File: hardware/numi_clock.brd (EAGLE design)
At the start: 70.8 x 29.5 mm, 31 parts, among them IC1 MEGA8-AI, IC2 LM75, Q1 12MHz, Y1 32.768kHz

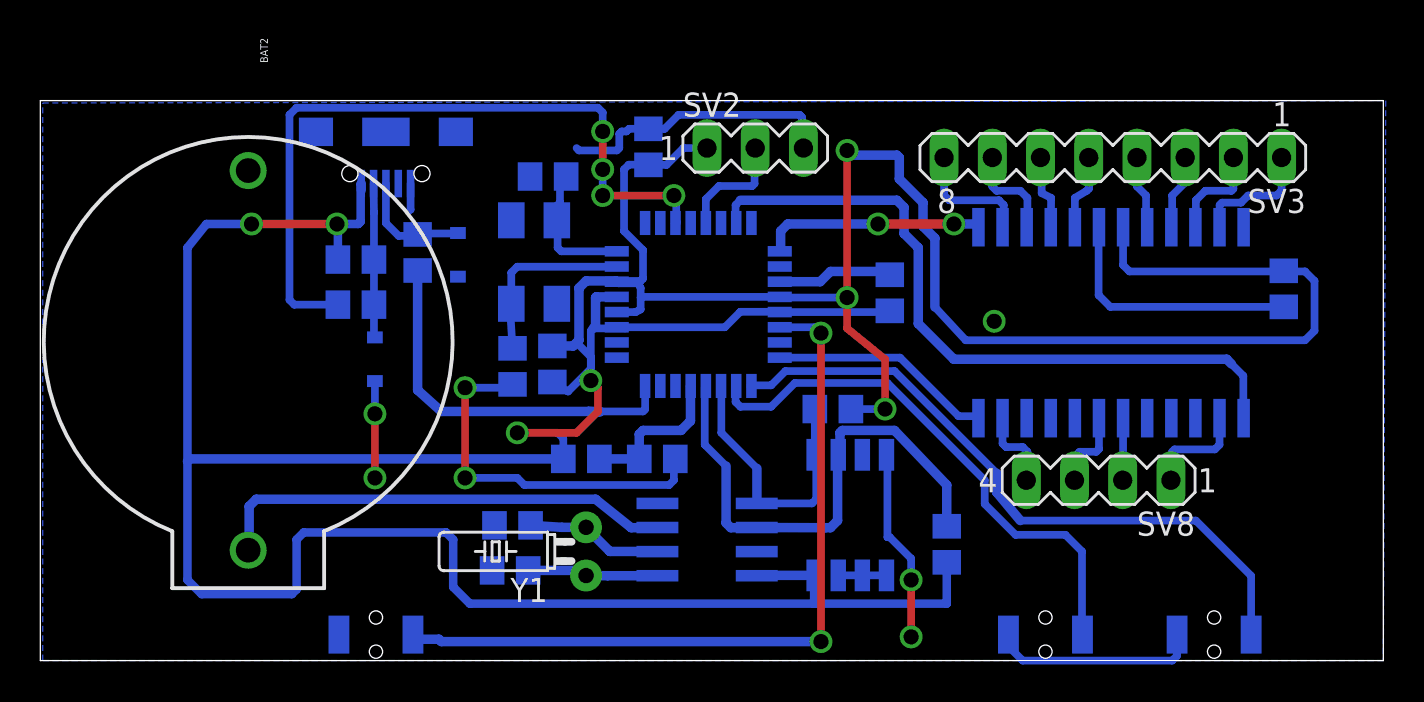
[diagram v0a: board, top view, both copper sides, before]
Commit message: rerouted some tracks
rerouted some tracks
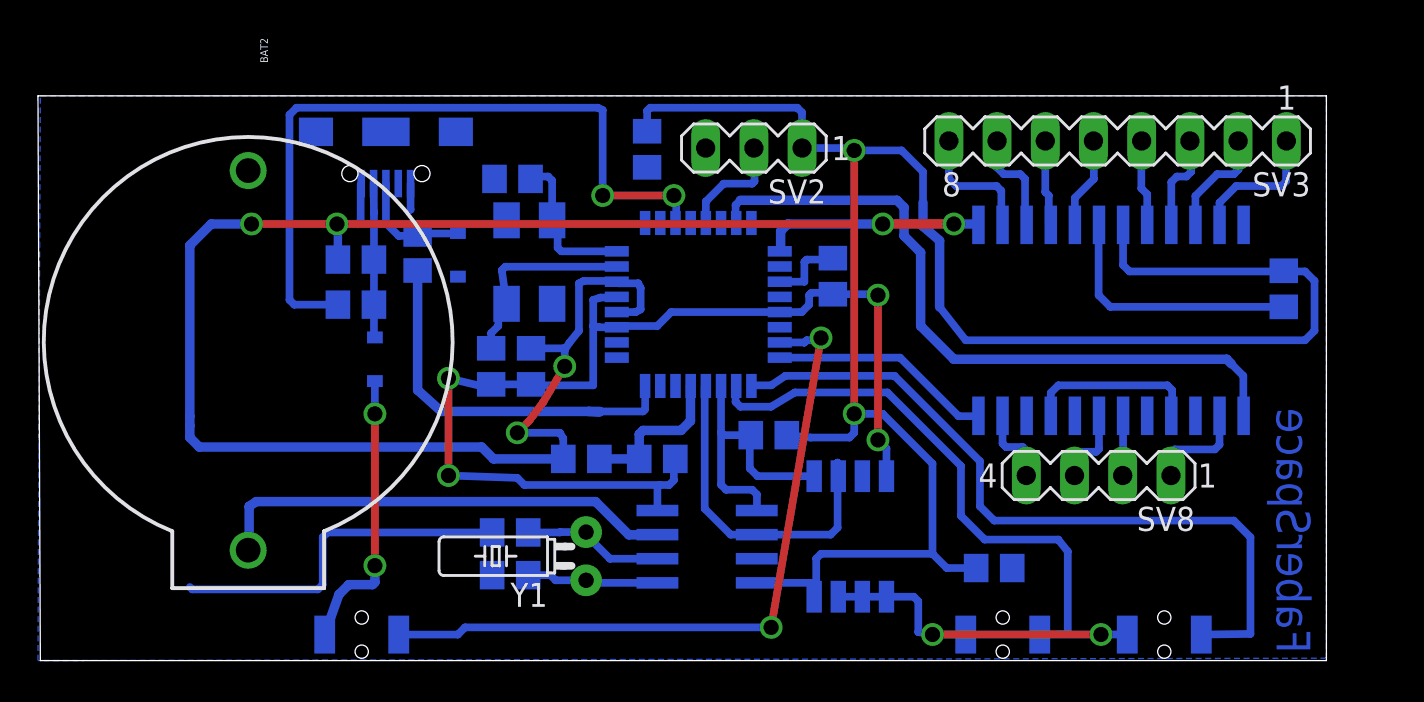
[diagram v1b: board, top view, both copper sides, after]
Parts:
- moved R8 3.64 mm to (53.5, 19.9)
- moved D3 3.12 mm to (56.9, 28.2)
- moved R10 2.80 mm to (65.4, 12.9), turned to 180 degrees
- moved S2 2.62 mm to (74.3, 9.37)
- moved S1 2.25 mm to (65.8, 9.37)
- moved C3 1.88 mm to (40.0, 33.4)
- moved C5 1.13 mm to (41.0, 23.5)
- moved C2 1.12 mm to (38.9, 23.5)
- moved IC2 1.12 mm to (57.2, 14.5)
- moved SV3 0.91 mm to (71.9, 35.4)
- moved S3 0.75 mm to (32.1, 9.37)
- moved C10 0.40 mm to (39.9, 14.8)
- moved U$2 0.38 mm to (50.2, 14.0)
- moved C9 0.25 mm to (39.9, 12.5)
- moved Q1 0.25 mm to (40.9, 29.0)
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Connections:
- net +5V: no longer IC1.20
- net FUNC: now also IC1.23; no longer IC1.22
- net SCL: no longer R10.2
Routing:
- net GND: track 89.6 -> 123.1 mm, vias 6 -> 8
- net +5V: track 216.8 -> 196.3 mm, vias 7 -> 6
- net SCL: track 27.6 -> 18.4 mm
- net MINUTE: track 34.9 -> 39.1 mm
- net FUNC: track 40.2 -> 37.5 mm
- net LED: track 6.09 -> 3.92 mm
- net F: track 3.97 -> 5.30 mm
- net N$4: track 8.21 -> 6.98 mm
- net N$1: track 9.69 -> 10.8 mm
- net N$2: track 7.10 -> 8.13 mm
- net DP: track 6.49 -> 7.48 mm
- net D: track 4.08 -> 5.05 mm
- net HOUR: track 28.7 -> 29.5 mm
- net E: track 3.89 -> 4.76 mm
- net G: track 5.30 -> 6.08 mm
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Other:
- board size 70.8 x 29.5 mm -> 67.9 x 29.8 mm
- board text added: "FaberSpace"
